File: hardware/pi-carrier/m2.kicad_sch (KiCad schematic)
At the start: 23 parts, among them J4 Bus_M.2_Socket_M, J7 Conn_01x16_MountingPin, U7 TPS563203

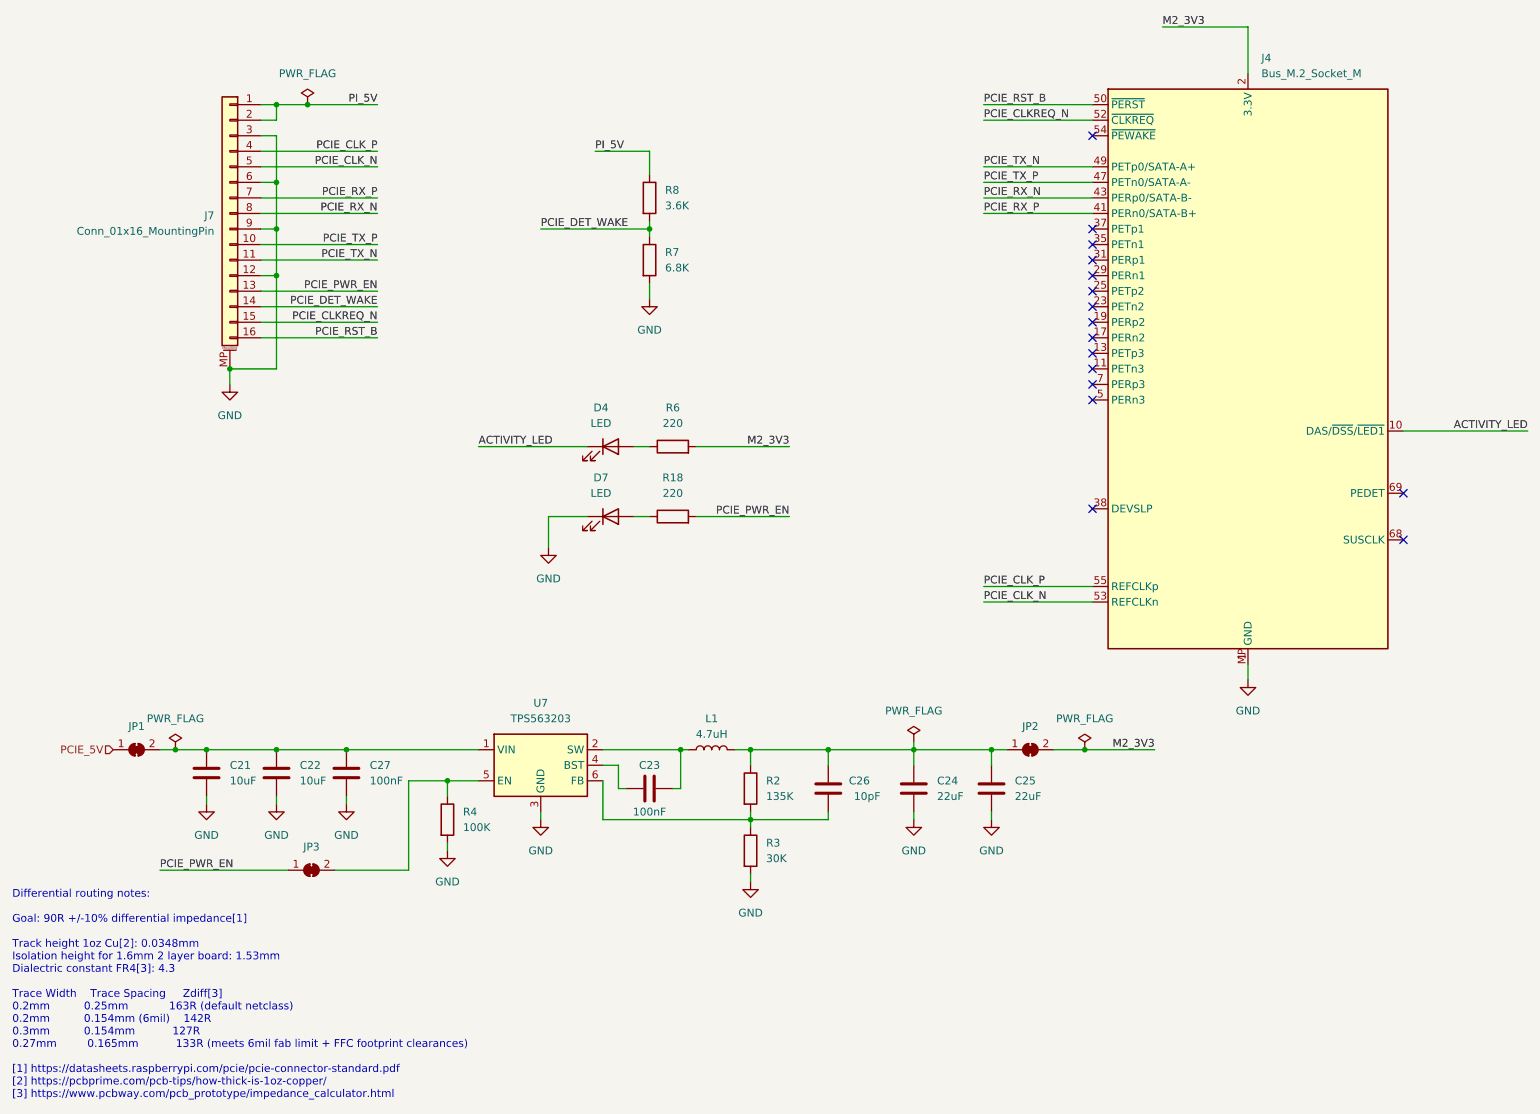
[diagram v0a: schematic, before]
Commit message: pi-carrier: drive EN LED from within block
Problem the EN LED is connected "outside" the jumper
but it is really part of the power supply block.

Connect it to the other end of the jumper.
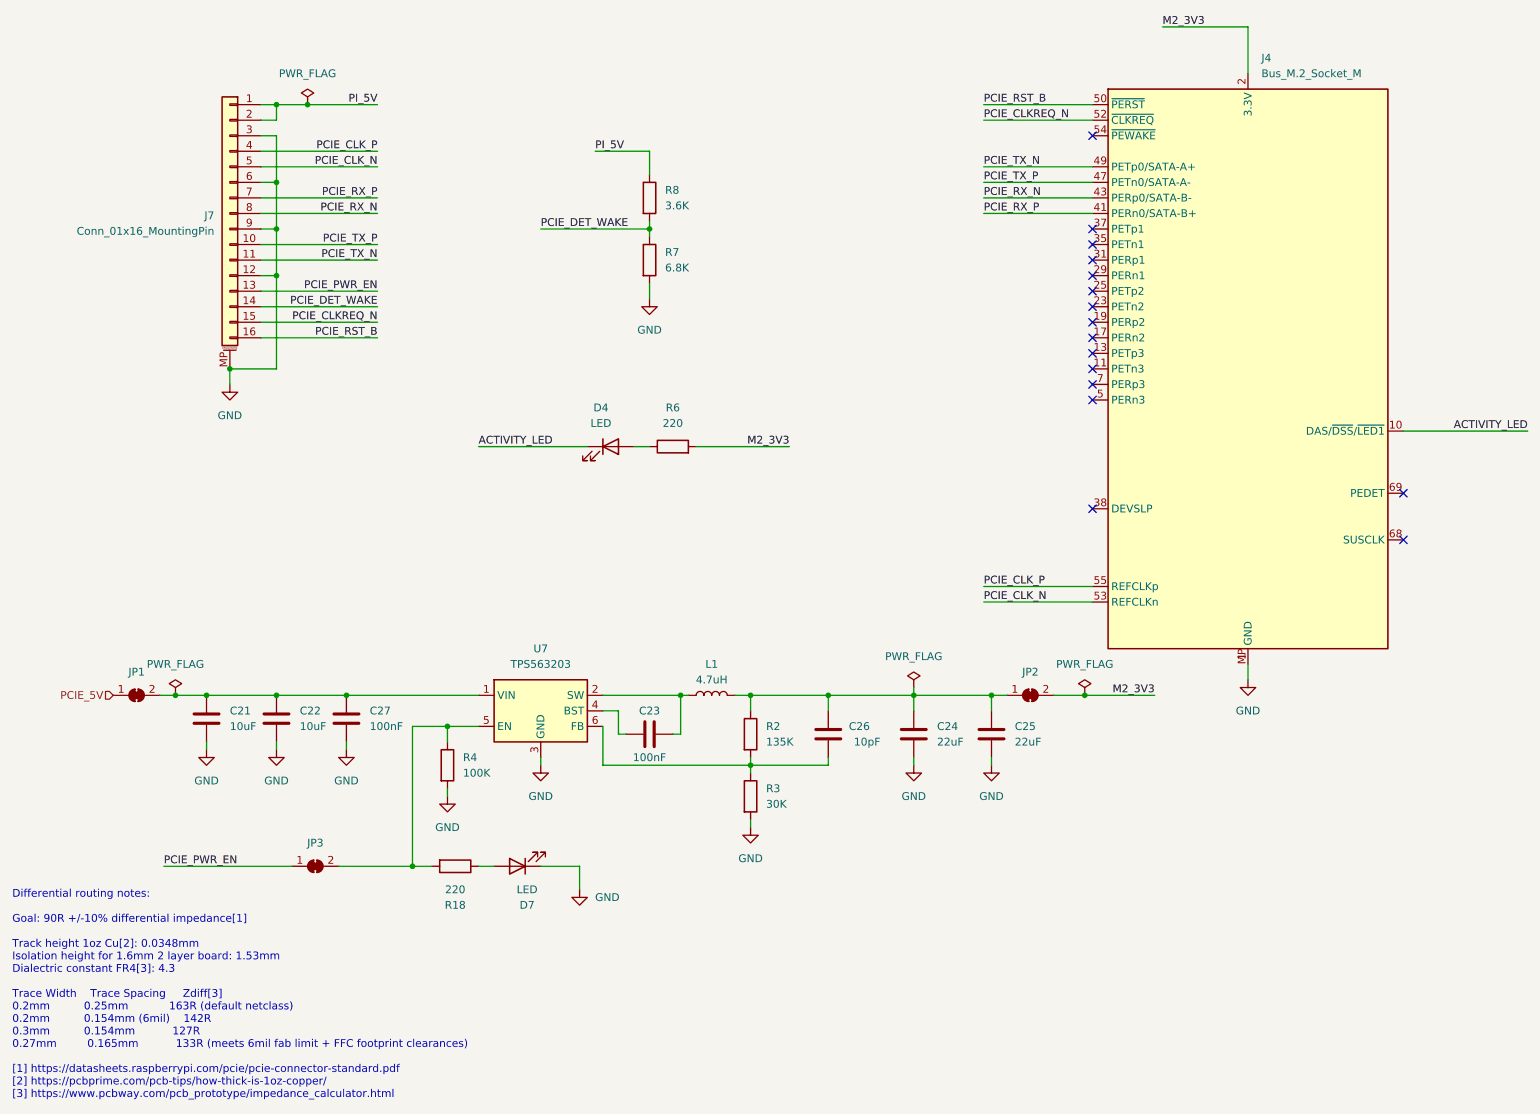
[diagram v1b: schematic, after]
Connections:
- net PCIE_PWR_EN: no longer R18.2
- net at JP3.2 (B), R4.1, U7.5 (EN): now also R18.2
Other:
- moved on the sheet: C21, C22, C23, C24, C25, C26, C27, D7, JP1, JP2, JP3, L1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
